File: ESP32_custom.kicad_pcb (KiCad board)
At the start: 4 copper layers, 26 parts, among them J1 TYPE-C-31-M-12, J2 Conn_01x16_Pin, J3 Conn_01x16_Pin, Q1 SS8050, Q2 SS8050, SW1 SW_Push, SW2 SW_Push, U2 ESP32-WROOM-32E 8MB, U3 CH340C, U4 AMS1117-3.3

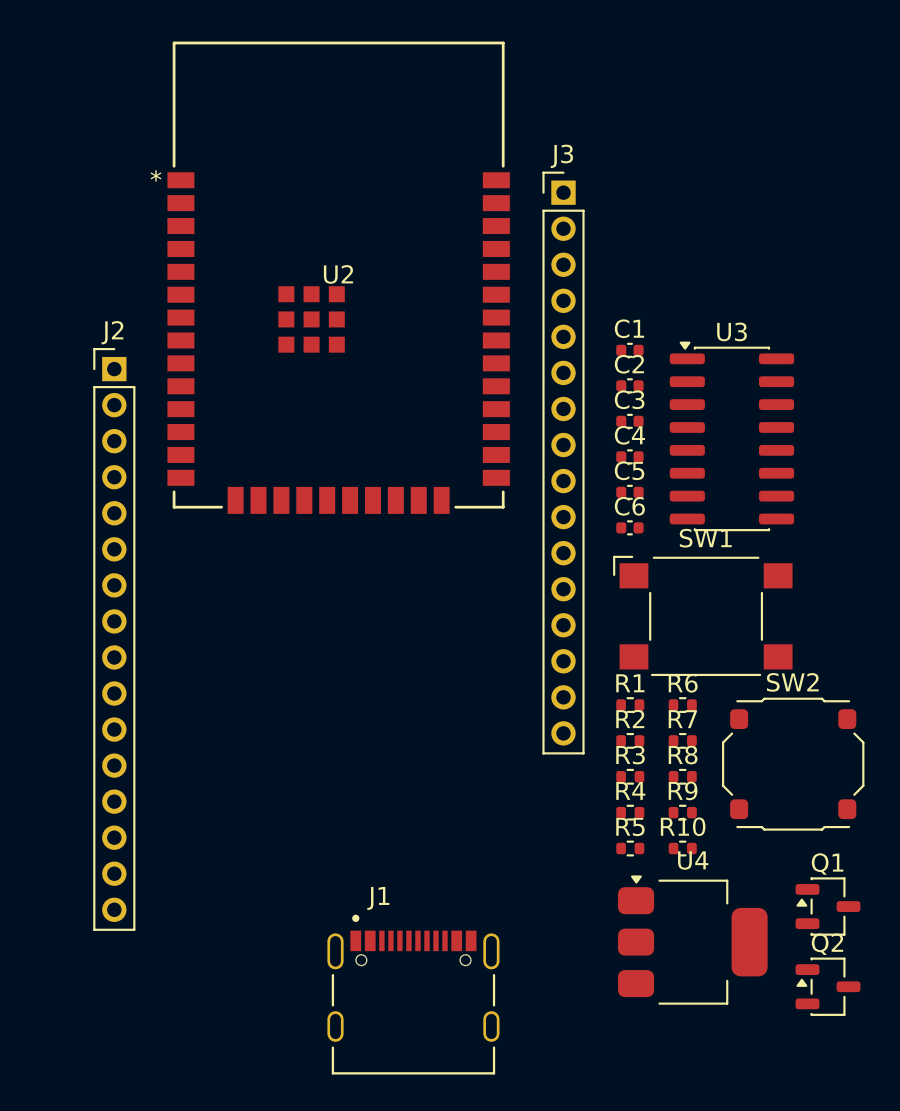
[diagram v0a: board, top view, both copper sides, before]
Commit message: arranging footprint
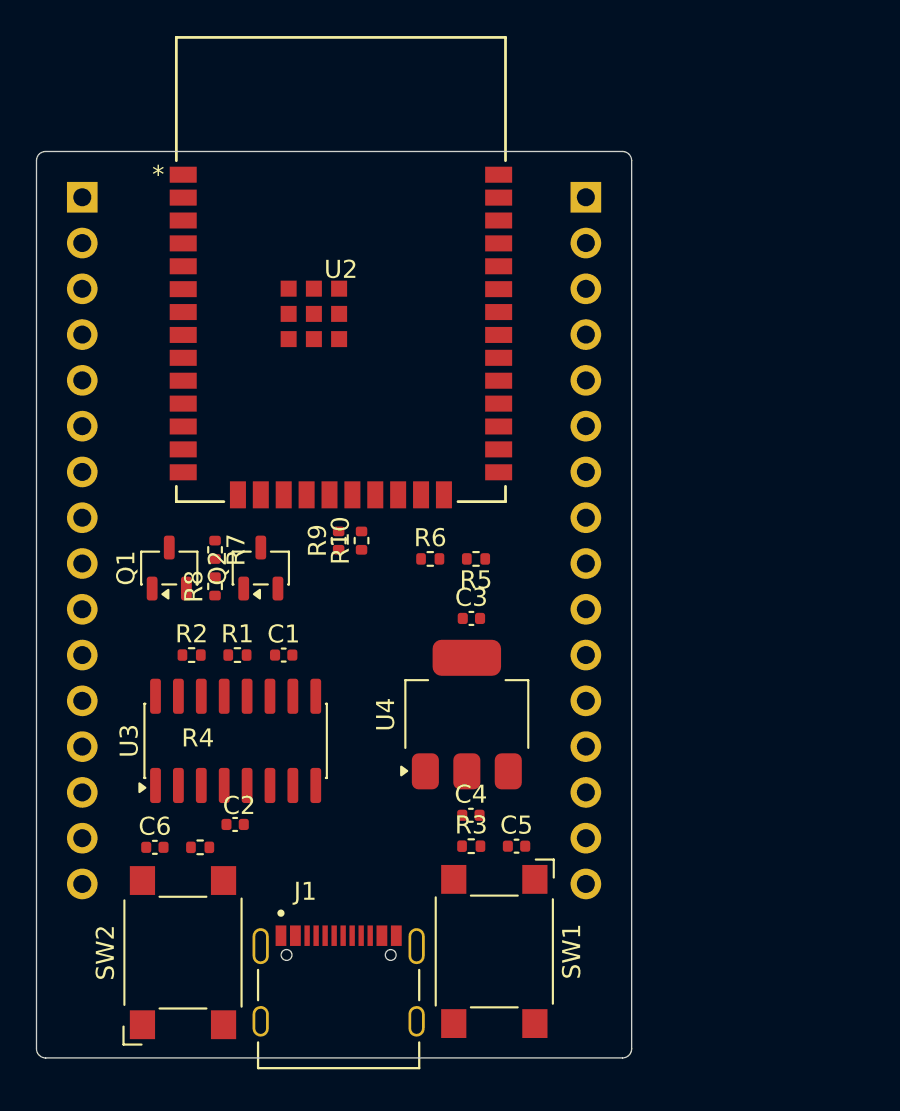
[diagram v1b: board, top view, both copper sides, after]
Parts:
- J2, J3: footprint Connector_PinHeader_2.00mm:PinHeader_1x16_P2.00mm_Vertical -> Connector_PinHeader_2.54mm:PinHeader_1x16_P2.54mm_Vertical; moved to B.Cu
- SW2: footprint Button_Switch_SMD:SW_SPST_GT-TC155X -> Button_Switch_SMD:SW_SPST_Omron_B3FS-100xP
- moved Q1 41.1 mm to (119.1, 83.6), turned to 90 degrees
- moved Q2 39.1 mm to (124.2, 83.6), turned to 90 degrees
- moved SW2 35.4 mm to (119.9, 104.9), turned to 90 degrees
- moved C2 32.7 mm to (122.8, 97.8)
- moved U3 32.2 mm to (122.8, 93.2), turned to 90 degrees
- moved C6 31.8 mm to (118.3, 99.1)
- moved R7 28.0 mm to (121.7, 82.6), turned to -90 degrees
- moved R8 28.0 mm to (121.7, 84.6), turned to 90 degrees
- moved C1 25.6 mm to (125.5, 88.4)
- moved R2 24.8 mm to (120.4, 88.4)
- moved R10 24.7 mm to (129.8, 82.0), turned to 90 degrees
- moved R9 24.3 mm to (128.5, 82.0), turned to 90 degrees
- moved R4 23.9 mm to (120.8, 99.1)
- moved SW1 22.0 mm to (137.2, 104.8), turned to -90 degrees
- moved R1 22.0 mm to (122.9, 88.4)
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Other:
- board outline added: 33 x 50.3 mm
